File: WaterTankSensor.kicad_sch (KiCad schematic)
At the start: 6 parts, among them U1 ESP32, U2 ESP32-S3-MINI-1

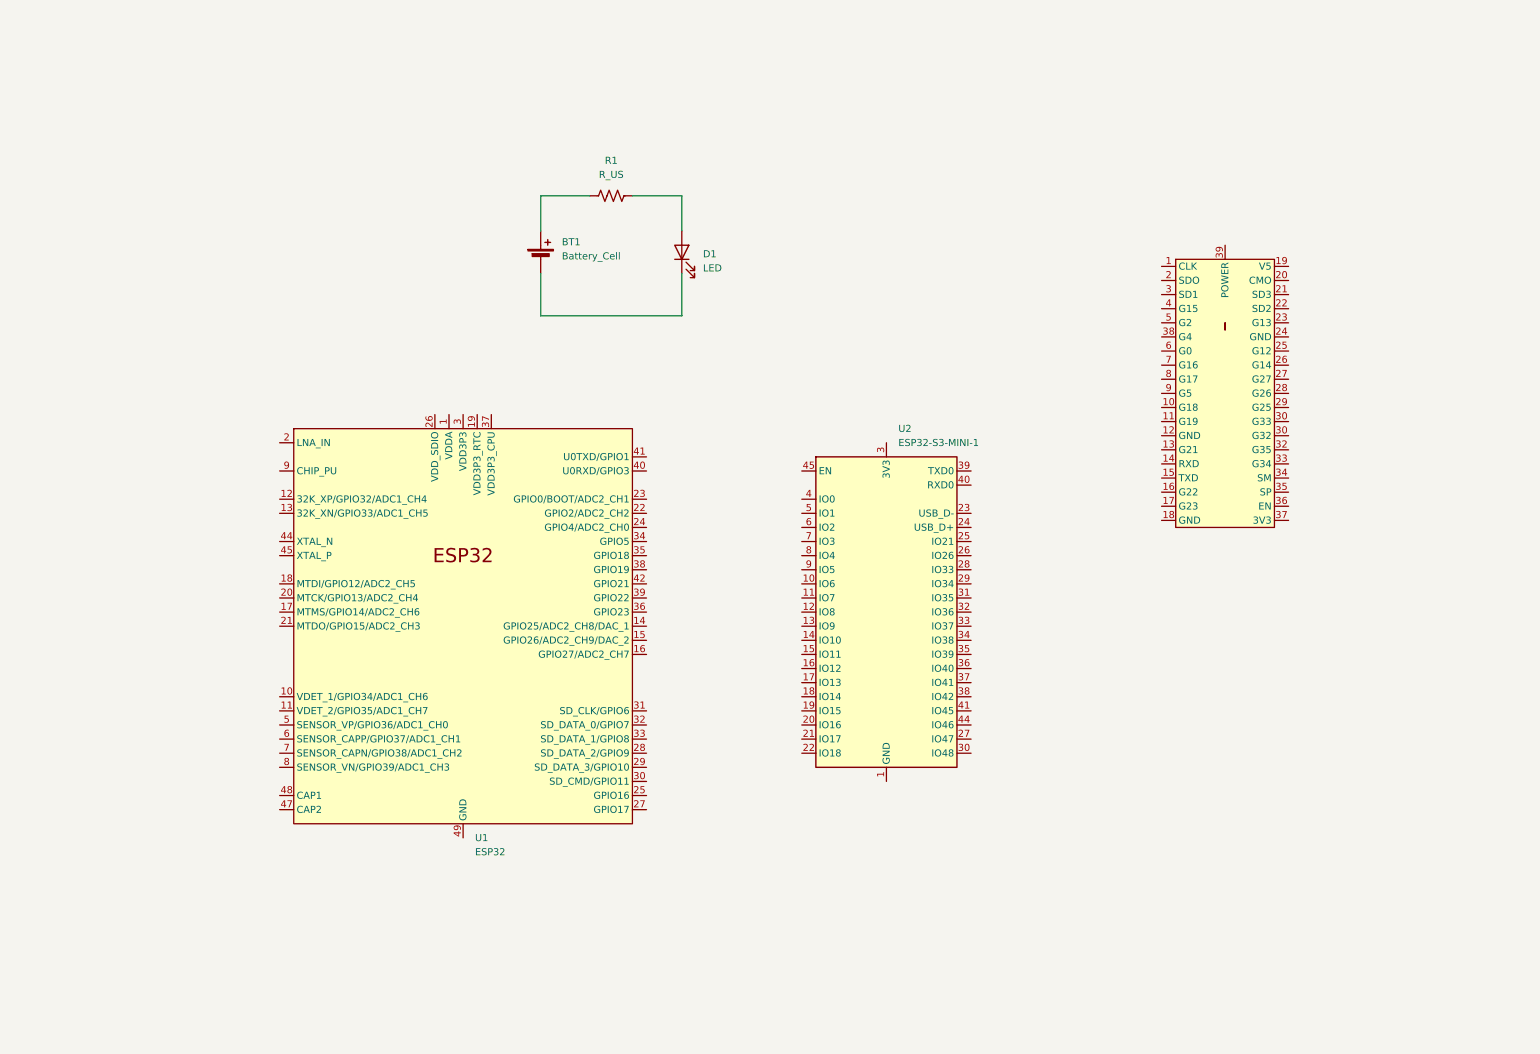
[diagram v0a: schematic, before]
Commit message: PowerSupply
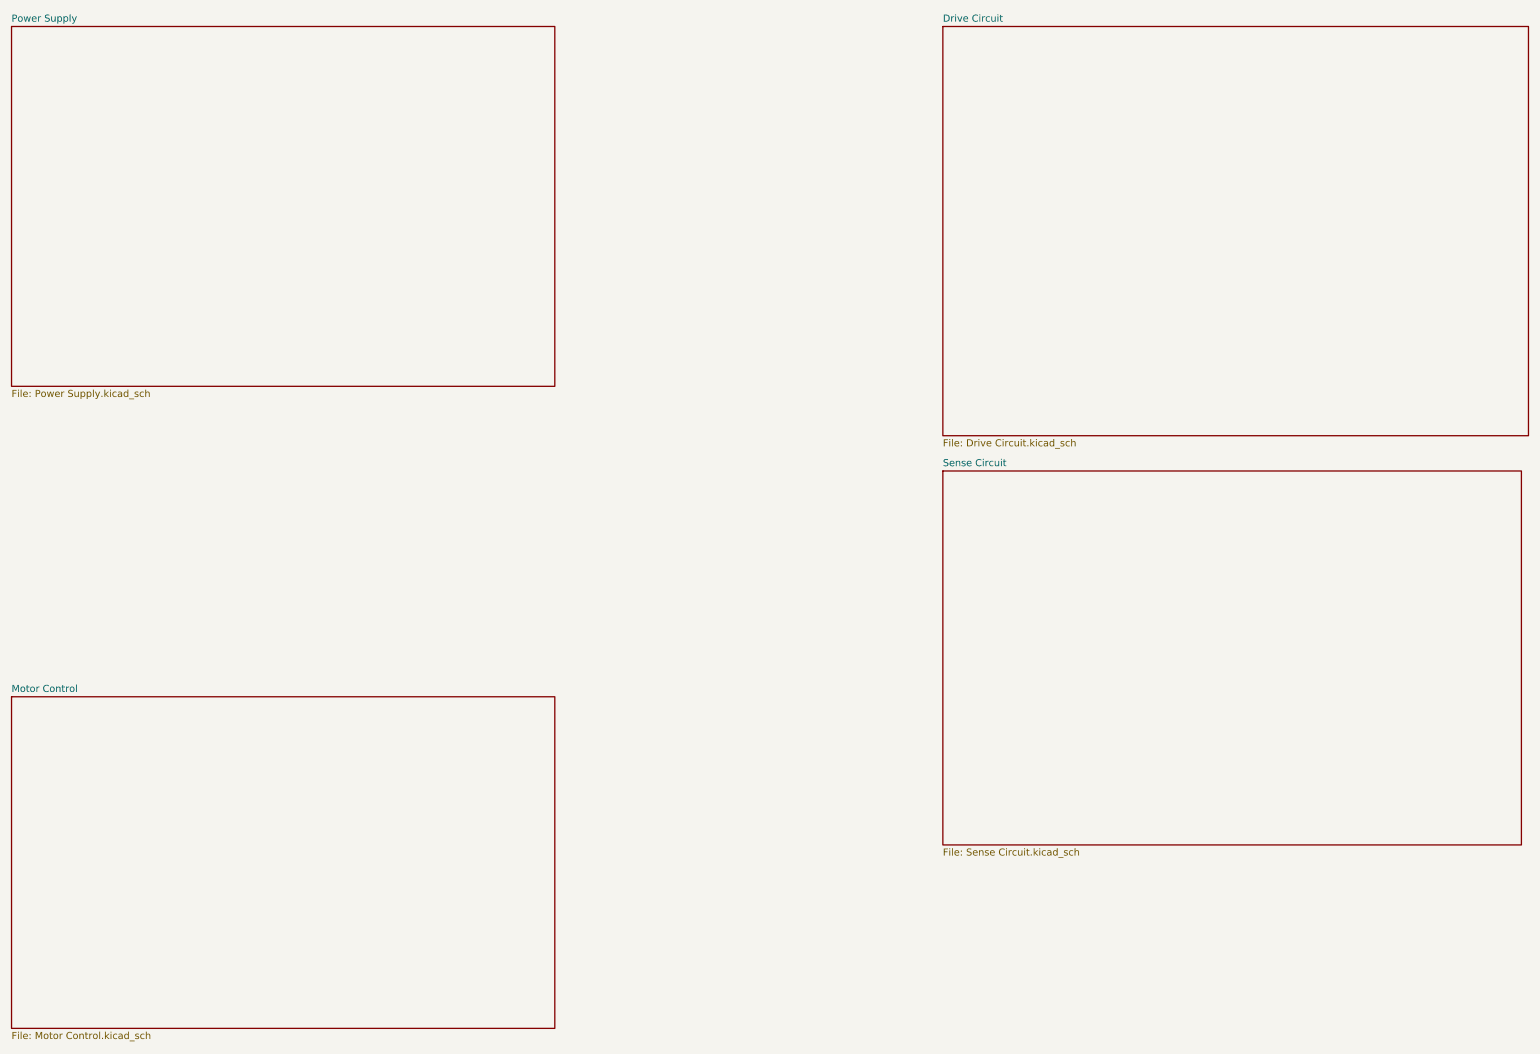
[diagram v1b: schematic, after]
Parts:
- removed BT1: Battery_Cell, symbol Device:Battery_Cell
- removed D1: LED, symbol Device:LED
- removed R1: R_US, symbol Device:R_US
- removed U1: ESP32, Package_DFN_QFN:QFN-48-1EP_6x6mm_P0.4mm_EP4.3x4.3mm, symbol PCM_Espressif:ESP32
- removed U2: ESP32-S3-MINI-1, RF_Module:ESP32-S2-MINI-1, symbol RF_Module:ESP32-S3-MINI-1
- removed U3: ~, symbol New_Library:ESP-nav
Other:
- added sheet Drive Circuit (Drive Circuit.kicad_sch)
- added sheet Motor Control (Motor Control.kicad_sch)
- added sheet Power Supply (Power Supply.kicad_sch)
- added sheet Sense Circuit (Sense Circuit.kicad_sch)
